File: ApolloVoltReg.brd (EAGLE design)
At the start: 42.8 x 26.7 mm, 27 parts, among them IC2 TL084D, J1 SSM-108-L-DV-BE-K-APOLLO, U1 TEXAS_INSTRUMENTS_PTH04070WAD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, U2 ACS712ELCTR-05B-T

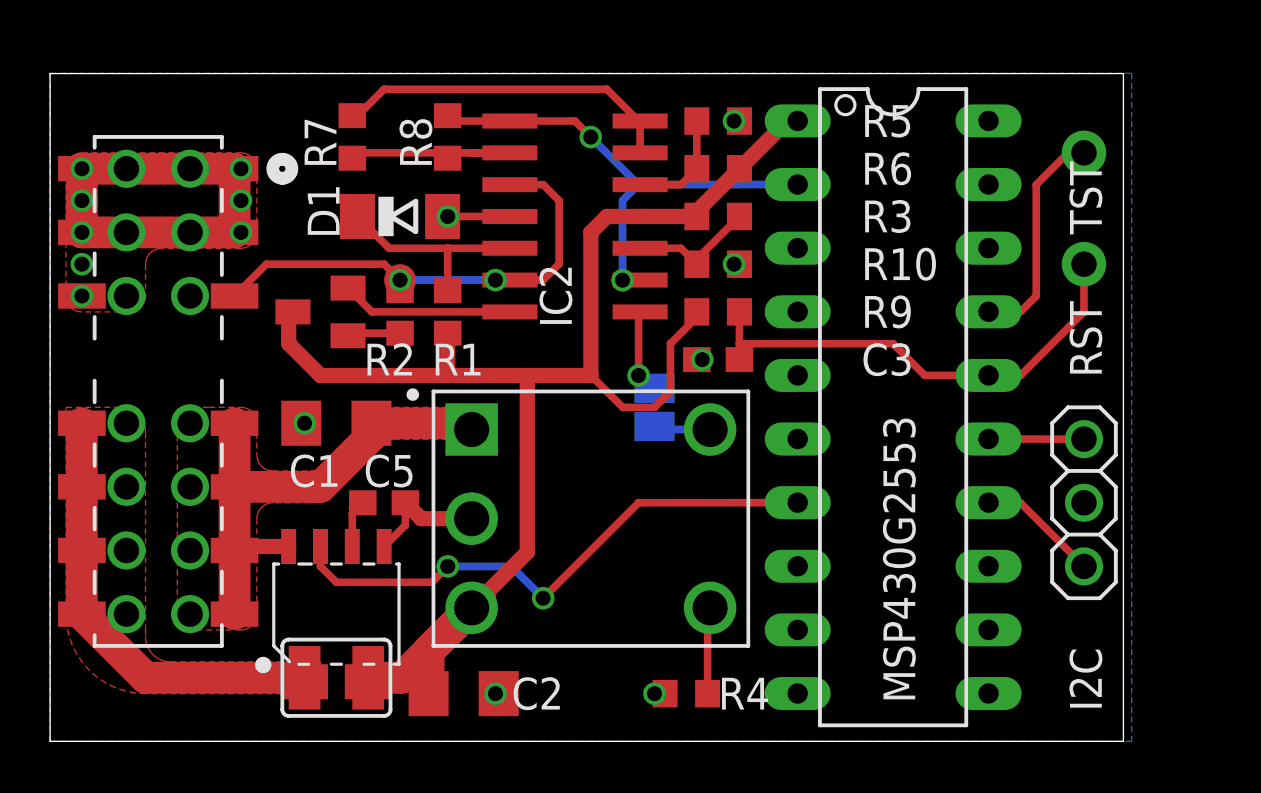
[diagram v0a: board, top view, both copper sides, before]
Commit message: gerber in archs
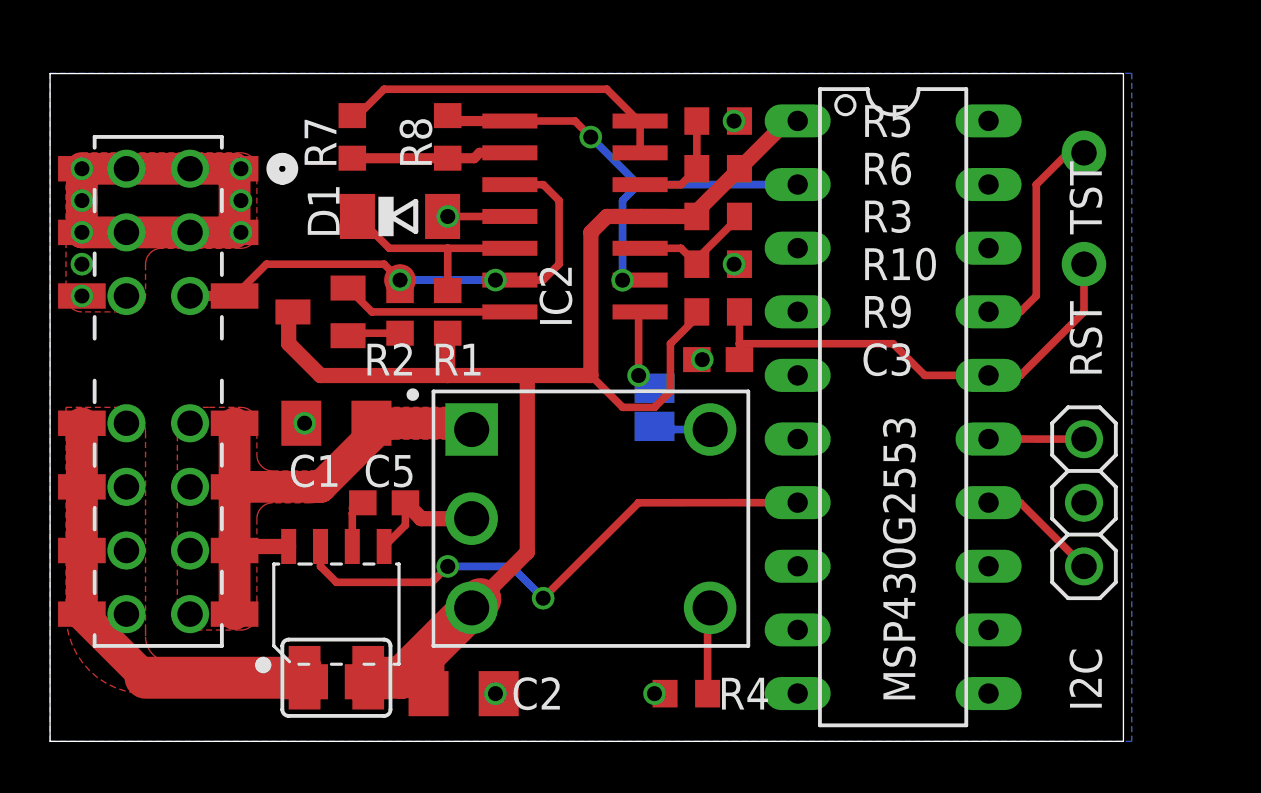
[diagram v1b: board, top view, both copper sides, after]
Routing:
- net THERM1: track 18.6 -> 20.4 mm
- net N$8: track 8.01 -> 6.38 mm
- net VCC: track 59.2 -> 60.7 mm
- net CPU: track 17.6 -> 19.0 mm
- net N$12: track 3.26 -> 4.11 mm
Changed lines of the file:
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@@
 <grid distance="0.025" unitdist="inch" unit="inch" style="lines" multiple="1" display="yes" altdistance="0.025" altunitdist="inch" altunit="inch"/>
 <layers>
-<layer number="1" name="Top" color="4" fill="1" visible="yes" active="yes"/>
-<layer number="16" name="Bottom" color="1" fill="1" visible="yes" active="yes"/>
+<layer number="1" name="Top" color="4" fill="1" visible="no" active="yes"/>
+<layer number="16" name="Bottom" color="1" fill="1" visible="no" active="yes"/>
 <layer number="17" name="Pads" color="2" fill="1" visible="yes" active="yes"/>
 <layer number="18" name="Vias" color="2" fill="1" visible="yes" active="yes"/>
@@
 ©2019 Szymon Biegański
 github.com/sq7bti/ApolloVR</text>
+<dimension x1="1.27" y1="0" x2="44.45" y2="0" x3="22.86" y3="-3.175" textsize="1.778" layer="20" dtype="horizontal"/>
+<dimension x1="1.27" y1="0" x2="1.27" y2="26.67" x3="-1.27" y3="13.335" textsize="1.778" layer="20" dtype="horizontal"/>
 </plain>
 <attributes>
@@
 <contactref element="THERM" pad="TP"/>
 <contactref element="J1" pad="25"/>
+<wire x1="6.858" y1="17.78" x2="8.636" y2="17.78" width="0.4064" layer="1"/>
 <wire x1="19.05" y1="18.415" x2="19.625" y2="18.415" width="0" layer="19" extent="1-1"/>
-<wire x1="6.858" y1="17.78" x2="8.636" y2="17.78" width="0" layer="19" extent="1-1"/>
 </signal>
 <signal name="+5V">
@@
 <contactref element="R7" pad="2"/>
 <contactref element="R8" pad="1"/>
-<wire x1="19.625" y1="23.495" x2="17.995" y2="23.495" width="0.3048" layer="1"/>
-<wire x1="19.625" y1="23.495" x2="13.55" y2="23.495" width="0.3048" layer="1"/>
-<wire x1="13.55" y1="23.495" x2="13.335" y2="23.28" width="0.3048" layer="1"/>
-<wire x1="17.995" y1="23.495" x2="17.145" y2="23.28" width="0" layer="19" extent="1-1"/>
+<wire x1="13.335" y1="23.28" x2="17.145" y2="23.28" width="0.4064" layer="1"/>
+<wire x1="17.145" y1="23.28" x2="18.2" y2="23.28" width="0.4064" layer="1"/>
+<wire x1="18.2" y1="23.28" x2="18.415" y2="23.495" width="0.4064" layer="1"/>
+<wire x1="18.415" y1="23.495" x2="19.625" y2="23.495" width="0.4064" layer="1"/>
 </signal>
 <signal name="TEMPSENS">
@@
 <contactref element="IC2" pad="8"/>
 <contactref element="MSP430G2553" pad="2"/>
-<wire x1="19.625" y1="24.765" x2="17.36" y2="24.765" width="0.3048" layer="1"/>
-<wire x1="17.36" y1="24.765" x2="17.145" y2="24.98" width="0.3048" layer="1"/>
 <wire x1="19.625" y1="24.765" x2="22.225" y2="24.765" width="0.3048" layer="1"/>
 <wire x1="22.225" y1="24.765" x2="22.855" y2="24.125" width="0.3048" layer="1"/>
@@
 <wire x1="24.755" y1="22.225" x2="24.125" y2="21.595" width="0.3048" layer="16"/>
 <wire x1="24.125" y1="21.595" x2="24.125" y2="18.41" width="0.3048" layer="16"/>
+<wire x1="19.625" y1="24.765" x2="17.36" y2="24.765" width="0.4064" layer="1"/>
+<wire x1="17.36" y1="24.765" x2="17.145" y2="24.98" width="0.4064" layer="1"/>
 <wire x1="24.125" y1="18.41" x2="24.825" y2="18.415" width="0" layer="19" extent="1-1"/>
 </signal>
@@
 <wire x1="17.145" y1="16.295" x2="17.145" y2="14.605" width="0.6096" layer="1"/>
 <wire x1="20.32" y1="14.605" x2="22.86" y2="14.605" width="0.6096" layer="1"/>
-<wire x1="13.97" y1="2.54" x2="15.31" y2="2.54" width="1.27" layer="1"/>
-<wire x1="15.31" y1="2.54" x2="18.45" y2="5.68" width="1.27" layer="1"/>
+<wire x1="13.97" y1="2.54" x2="15.31" y2="2.54" width="1.6764" layer="1"/>
+<wire x1="15.31" y1="2.54" x2="18.45" y2="5.68" width="1.6764" layer="1"/>
 <contactref element="R3" pad="2"/>
 <wire x1="24.825" y1="20.955" x2="23.495" y2="20.955" width="0.6096" layer="1"/>
@@
 <wire x1="25.4" y1="13.335" x2="24.13" y2="13.335" width="0.3048" layer="1"/>
 <wire x1="24.13" y1="13.335" x2="22.86" y2="14.605" width="0.3048" layer="1"/>
-<wire x1="13.335" y1="2.38" x2="13.97" y2="2.54" width="0" layer="19" extent="1-1"/>
-<wire x1="14.605" y1="2.38" x2="13.97" y2="2.54" width="0" layer="19" extent="1-1"/>
+<wire x1="13.335" y1="2.38" x2="13.97" y2="2.38" width="0.4064" layer="1"/>
+<wire x1="14.605" y1="2.38" x2="13.97" y2="2.38" width="0.4064" layer="1"/>
+<wire x1="13.97" y1="2.38" x2="13.97" y2="2.54" width="0.4064" layer="1"/>
 </signal>
 <signal name="CPU">
@@
 <wire x1="2.54" y1="12.7" x2="2.54" y2="5.08" width="1.27" layer="1"/>
 <wire x1="2.54" y1="5.08" x2="5.08" y2="2.54" width="1.27" layer="1"/>
-<wire x1="5.08" y1="2.54" x2="11.43" y2="2.54" width="1.27" layer="1"/>
+<wire x1="5.08" y1="2.54" x2="11.43" y2="2.54" width="1.6764" layer="1"/>
 <polygon width="0.4064" layer="1">
 <vertex x="1.905" y="13.335"/>
@@
 <contactref element="J1" pad="34"/>
 <contactref element="J1" pad="36"/>
-<wire x1="11.43" y1="2.54" x2="10.795" y2="2.38" width="0" layer="19" extent="1-1"/>
-<wire x1="12.065" y1="2.38" x2="11.43" y2="2.54" width="0" layer="19" extent="1-1"/>
+<wire x1="10.795" y1="2.38" x2="11.43" y2="2.38" width="0.4064" layer="1"/>
+<wire x1="12.065" y1="2.38" x2="11.43" y2="2.38" width="0.4064" layer="1"/>
+<wire x1="11.43" y1="2.38" x2="11.43" y2="2.54" width="0.4064" layer="1"/>
 </signal>
 <signal name="N$9">
@@
 <wire x1="24.765" y1="14.605" x2="24.765" y2="17.085" width="0.3048" layer="1"/>
 <wire x1="24.765" y1="17.085" x2="24.825" y2="17.145" width="0.3048" layer="1"/>
-<wire x1="24.765" y1="14.605" x2="25.4" y2="14.097" width="0" layer="19" extent="16-16"/>
+<wire x1="25.4" y1="14.097" x2="25.273" y2="14.097" width="0.4064" layer="16"/>
+<wire x1="25.273" y1="14.097" x2="24.765" y2="14.605" width="0.4064" layer="16"/>
 </signal>
 </signals>

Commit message: adding pic
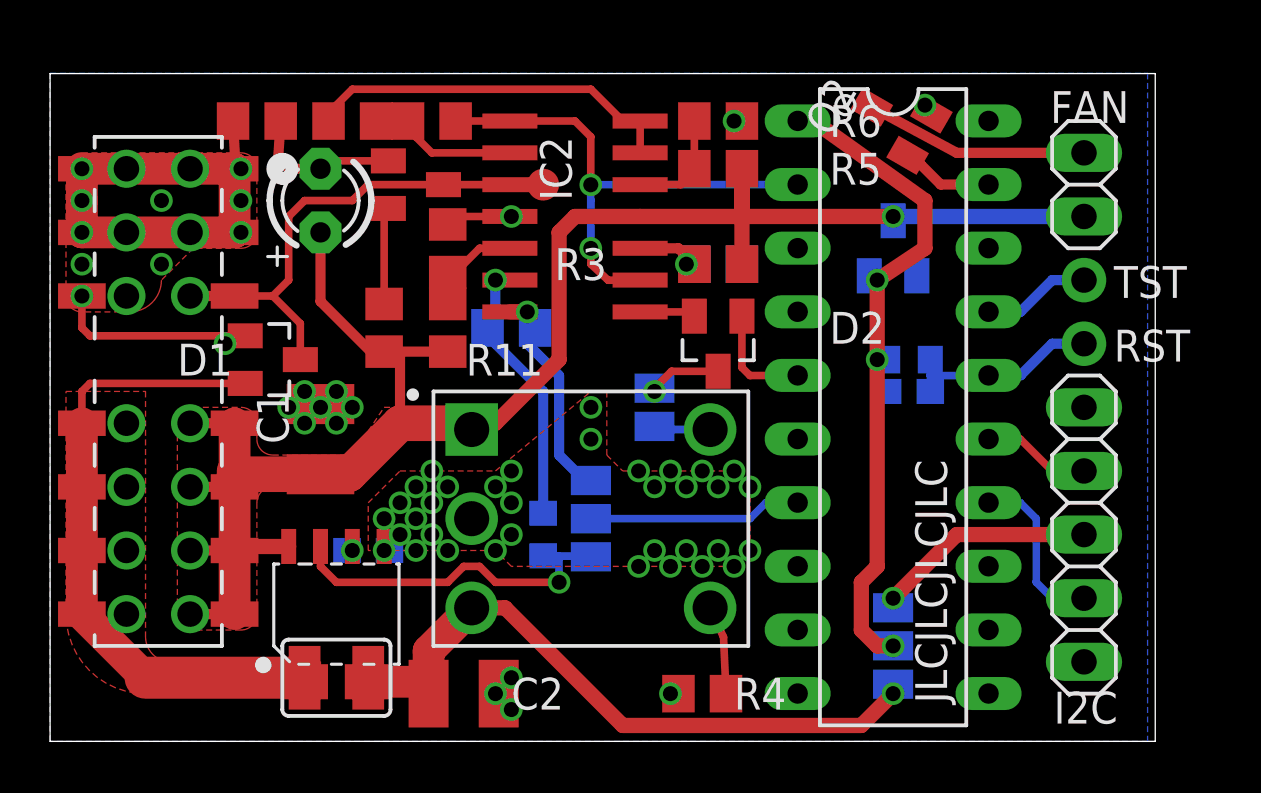
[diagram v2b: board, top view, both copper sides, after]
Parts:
- removed T1: (no value), transistor:SOT23-EBC
- added D2: BAS40-06, diode:SOT23
- added FAN: (no value), pinhead:1X02
- added IC1: MCP1703CB, linear:SOT23
- added LED1: (no value), adafruit:LED3MM
- added Q1: (no value), semicon-smd-ipc:SOT23
- added Q2: (no value), adafruit:SOT23
- added R11, R12, R13: 2k, resistor:R0805
- added R14: 2k, resistor:R0603
- added SJ3, SJ5: (no value), jumper:SJ_2
- C1, C2: device eagle-ltspice:C1206 -> eagle-ltspice:C1210
- D1: value (none) -> BAS40-04; device diode:SOD80C -> diode:SOT23
- I2C: device adafruit:1X03 -> pinhead:1X05
- R1: value 121 -> 1k; device resistor:R0603 -> resistor:R0805
- R10, R3, R4, R5, R6, R7, R8: device resistor:R0603 -> resistor:R0805
- R2: value 840 -> 1k3; device resistor:R0603 -> resistor:R0805
- moved R1 10.8 mm to (9.53, 24.8), turned to 180 degrees
- moved R9 7.85 mm to (35.6, 15.2), flipped to the bottom, turned to 180 degrees
- moved C3 7.73 mm to (35.6, 14.0), flipped to the bottom, turned to 0 degrees
- moved D1 7.65 mm to (10.2, 15.2), turned to 270 degrees
- moved THERM 6.87 mm to (21.0, 22.2)
- moved TST 5.08 mm to (42.5, 18.4)
- moved RST 3.18 mm to (42.5, 15.9)
- moved C5 2.01 mm to (14.0, 7.62), flipped to the bottom, turned to 0 degrees
- moved R3 1.90 mm to (27.9, 19.1), turned to 0 degrees
- moved I2C 1.27 mm to (42.5, 8.26)
- moved C1 0.90 mm to (12.1, 12.1), turned to 90 degrees
- moved R8 0.90 mm to (16.5, 24.8), turned to 0 degrees
- moved R2 0.90 mm to (14.6, 16.5)
- moved R7 0.64 mm to (13.3, 24.8), turned to 0 degrees
- moved R4 0.63 mm to (27.3, 1.91)
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- renumbered MSP430G2553 to JLCJLCJLCJLC
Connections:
- net N$9 renamed RST
- new net N$13: IC2.13, R11.2, R14.2
- new net N$14: IC2.14, R11.1, SJ3.1
- new net N$15: JLCJLCJLCJLC.7, SJ3.2
- new net N$16: IC1.2, JLCJLCJLCJLC.1, R9.1, SJ5.2
- new net N$17: D2.2, IC2.1
- new net N$18: D2.3, SJ2.1
- new net N$19: FAN.2, Q2.3
- new net N$21: I2C.3, SJ5.3
- new net N$9: JLCJLCJLCJLC.19, Q2.1
- net +5V: now also FAN.1, IC1.3, IC2.4, LED1.A, R12.1, R2.2, R3.2, R5.1
- net ACS_OUT: now also R14.1, SJ3.3; no longer JLCJLCJLCJLC.7
- net CPU: now also D1.2
- net GND: now also D1.1, I2C.1, I2C.5, IC1.1, Q2.2, R1.2, R13.2; no longer D1.A, I2C.2
- net N$12: now also D2.1, JLCJLCJLCJLC.5; no longer IC2.1, SJ2.1
- net N$2: now also LED1.K, Q1.1, R1.1; no longer D1.C, IC2.12, R1.2
- net N$3: now also Q1.2, R2.1; no longer IC2.14, T1.B
- net N$4: now also IC2.12, R12.2, R13.1; no longer R2.2, T1.E
- net SCL: now also I2C.4; no longer I2C.3
- net SDA: now also I2C.2; no longer I2C.1
- net THERM1: now also D1.3, Q1.3; no longer IC2.13, R2.1
- net VCC: now also SJ5.1; no longer IC2.4, JLCJLCJLCJLC.1, R1.1, R3.2, R5.1, R9.1, T1.C
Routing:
- net +5V: track 21.1 -> 76.3 mm, vias 0 -> 1
- net VCC: track 60.7 -> 27.2 mm, vias 0 -> 1
- net N$16: track 0.00 -> 26.9 mm, vias 0 -> 3
- net N$13: track 0.00 -> 11.4 mm, vias 0 -> 1
- net RST: track 19.1 -> 7.93 mm
- net N$14: track 0.00 -> 10.6 mm, vias 0 -> 1
- net N$21: track 0.00 -> 9.05 mm, vias 0 -> 1
- net N$19: track 0.00 -> 8.93 mm
- net N$15: track 0.00 -> 8.52 mm
- net ACS_OUT: track 22.5 -> 14.1 mm, vias 2 -> 1
- net CPU: track 19.0 -> 26.9 mm
- net GND: track 25.0 -> 31.8 mm, vias 15 -> 60
- net N$10: track 9.04 -> 4.33 mm
- net N$9: track 0.00 -> 3.69 mm
- net N$18: track 0.00 -> 3.07 mm, vias 0 -> 1
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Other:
- board size 42.8 x 26.7 mm -> 44.1 x 26.7 mm
